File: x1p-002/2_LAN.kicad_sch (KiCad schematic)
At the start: 54 parts, among them U1 LAN9514, U5 M93C86-WMN6TP, X1 25MHz

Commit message: annotated everything with LCSC IDs
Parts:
- C10, C9: LCSC (none) -> C1557
- C12, C13, C14, C15, C16, C17, C18, C21, C22, C23, C24, C25, C26, C27, C28, C48: LCSC (none) -> C1525
- C29: LCSC (none) -> C52923
- R10, R12, R34: LCSC (none) -> C25744
- R11: footprint Capacitor_SMD:C_0402_1005Metric -> Resistor_SMD:R_0402_1005Metric; LCSC (none) -> C25752
- R28, R29, R31, R32, R33: LCSC (none) -> C17168
- R6: LCSC (none) -> C26083
- R8: LCSC (none) -> C25077
- TP4, TP5: now left out of the parts list
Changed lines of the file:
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@@
 			)
 		)
-		(property "Footprint" "Capacitor_SMD:C_0402_1005Metric"
+		(property "Footprint" "Resistor_SMD:R_0402_1005Metric"
 			(at 55.88 58.42 0)
 			(effects
@@
 			)
 		)
-		(property "LCSC" ""
+		(property "LCSC" "C25752"
 			(at 53.7718 54.4322 0)
 			(effects
@@
 			)
 		)
-		(property "LCSC" ""
+		(property "LCSC" "C1525"
 			(at 29.464 16.5608 0)
 			(effects
@@
 			)
 		)
-		(property "LCSC" ""
+		(property "LCSC" "C1525"
 			(at 53.1876 16.4084 0)
 			(effects
@@
 			)
 		)
-		(property "LCSC" ""
+		(property "LCSC" "C25744"
 			(at 54.61 123.5456 0)
 			(effects
@@
 			)
 		)
-		(property "LCSC" ""
+		(property "LCSC" "C1525"
 			(at 173.99 16.5608 0)
 			(effects
@@
 			)
 		)
-		(property "LCSC" ""
+		(property "LCSC" "C1557"
 			(at 23.876 91.7956 0)
 			(effects
@@
 			)
 		)
-		(property "LCSC" ""
+		(property "LCSC" "C1525"
 			(at 181.61 16.5608 0)
 			(effects
@@
 			)
 		)
-		(property "LCSC" ""
+		(property "LCSC" "C1525"
 			(at 189.23 16.5608 0)
 			(effects
@@
 			)
 		)
-		(property "LCSC" ""
+		(property "LCSC" "C52923"
 			(at 40.9956 55.4228 0)
 			(effects
@@
 			)
 		)
-		(property "LCSC" ""
+		(property "LCSC" "C17168"
 			(at 174.1889 182.88 0)
 			(effects
@@
 			)
 		)
-		(property "LCSC" ""
+		(property "LCSC" "C1525"
 			(at 219.71 173.3042 0)
 			(effects
@@
 		(unit 1)
 		(exclude_from_sim no)
-		(in_bom yes)
+		(in_bom no)
 		(on_board yes)
 		(dnp no)
@@
 			)
 		)
-		(property "LCSC" ""
+		(property "LCSC" "C1557"
 			(at 23.2156 74.0156 0)
 			(effects
@@
 			)
 		)
-		(property "LCSC" ""
+		(property "LCSC" "C26083"
 			(at 47.498 88.8238 0)
 			(effects
@@
 			)
 		)
-		(property "LCSC" ""
+		(property "LCSC" "C17168"
 			(at 154.94 152.5989 0)
 			(effects
@@
 			)
 		)
-		(property "LCSC" ""
+		(property "LCSC" "C1525"
 			(at 45.212 16.5608 0)
 			(effects
@@
 			)
 		)
-		(property "LCSC" ""
+		(property "LCSC" "C17168"
 			(at 57.15 129.7389 0)
 			(effects
@@
 			)
 		)
-		(property "LCSC" ""
+		(property "LCSC" "C25077"
 			(at 245.5926 24.257 0)
 			(effects
@@
 			)
 		)
-		(property "LCSC" ""
+		(property "LCSC" "C1525"
 			(at 196.85 16.5608 0)
 			(effects
@@
 			)
 		)
-		(property "LCSC" ""
+		(property "LCSC" "C1525"
 			(at 16.51 28.5242 0)
 			(effects
@@
 			)
 		)
-		(property "LCSC" ""
+		(property "LCSC" "C17168"
 			(at 57.15 142.0411 0)
 			(effects
@@
 			)
 		)
-		(property "LCSC" ""
+		(property "LCSC" "C17168"
 			(at 60.96 48.4589 0)
 			(effects
@@
 		(unit 1)
 		(exclude_from_sim no)
-		(in_bom yes)
+		(in_bom no)
 		(on_board yes)
 		(dnp no)
@@
 			)
 		)
-		(property "LCSC" ""
+		(property "LCSC" "C25744"
 			(at 167.8389 182.88 0)
 			(effects
@@
 			)
 		)
-		(property "LCSC" ""
+		(property "LCSC" "C1525"
 			(at 21.59 16.5608 0)
 			(effects
@@
 			)
 		)
-		(property "LCSC" ""
+		(property "LCSC" "C1525"
 			(at 158.75 16.5608 0)
 			(effects
@@
 			)
 		)
-		(property "LCSC" ""
+		(property "LCSC" "C1525"
 			(at 24.13 28.5242 0)
 			(effects
@@
 			)
 		)
-		(property "LCSC" ""
+		(property "LCSC" "C1525"
 			(at 151.13 16.5608 0)
 			(effects
@@
 			)
 		)
-		(property "LCSC" ""
+		(property "LCSC" "C1525"
 			(at 166.37 16.5608 0)
 			(effects
@@
 			)
 		)
-		(property "LCSC" ""
+		(property "LCSC" "C1525"
 			(at 40.64 40.9956 0)
 			(effects
@@
 			)
 		)
-		(property "LCSC" ""
+		(property "LCSC" "C1525"
 			(at 37.338 16.5608 0)
 			(effects
@@
 			)
 		)
-		(property "LCSC" ""
+		(property "LCSC" "C25744"
 			(at 54.9656 143.3576 0)
 			(effects

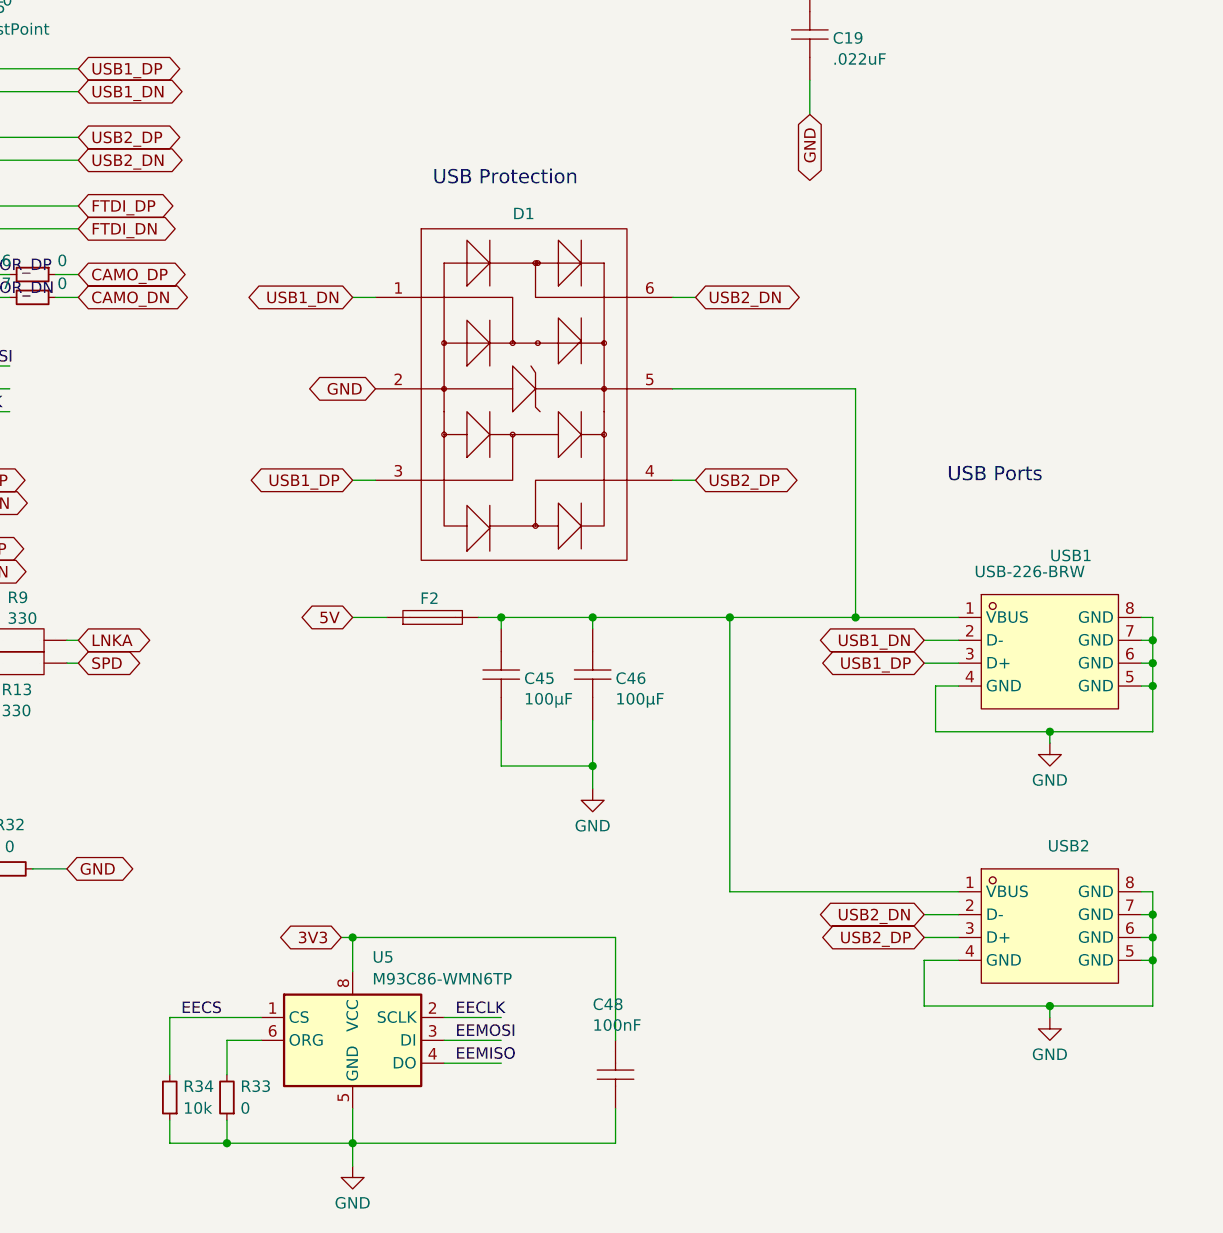
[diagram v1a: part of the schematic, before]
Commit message: stub-free usb esd protection
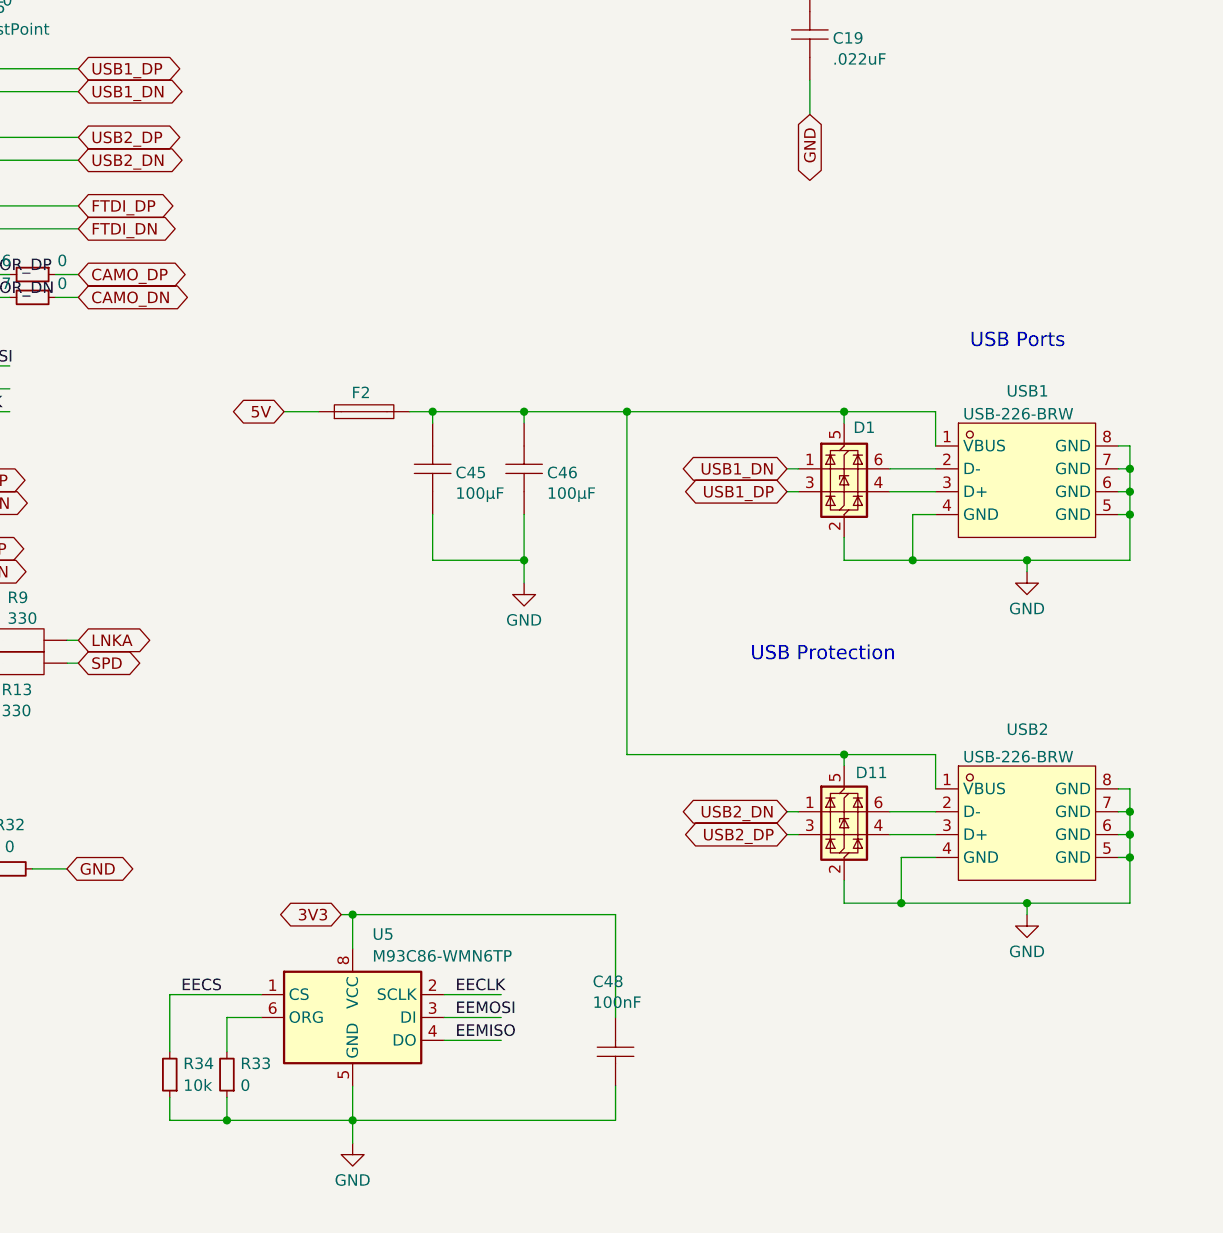
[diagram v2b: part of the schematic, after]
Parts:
- removed D1: SRV05-4.TCT_C2687126, x1-expander:SOT-23-6_L2.9-W1.6-P0.95-LS2.8-BL, symbol x1-expander:SRV05-4.TCT_C2687126
- added D1, D11: USBLC6-2SC6, Package_TO_SOT_SMD:SOT-23-6, symbol Power_Protection:USBLC6-2SC6
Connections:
- net GND: now also D1.2 (GND), D11.2 (GND)
- net USB1_DN: now also D1.1 (I/O1); no longer USB1.2 (D-)
- net USB1_DP: now also D1.3 (I/O2); no longer USB1.3 (D+)
- net USB2_DN: now also D11.1 (I/O1); no longer USB2.2 (D-)
- net USB2_DP: now also D11.3 (I/O2); no longer USB2.3 (D+)
- net at C45.2, C46.2, F2.2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: now also D1.5 (VBUS), D11.5 (VBUS)
- new net: D11.4 (I/O2), USB2.3 (D+)
- new net: D11.6 (I/O1), USB2.2 (D-)
- new net: D1.4 (I/O2), USB1.3 (D+)
- new net: D1.6 (I/O1), USB1.2 (D-)
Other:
- moved on the sheet: C45, C46, C48, F2, R33, R34, U5, USB1, USB2

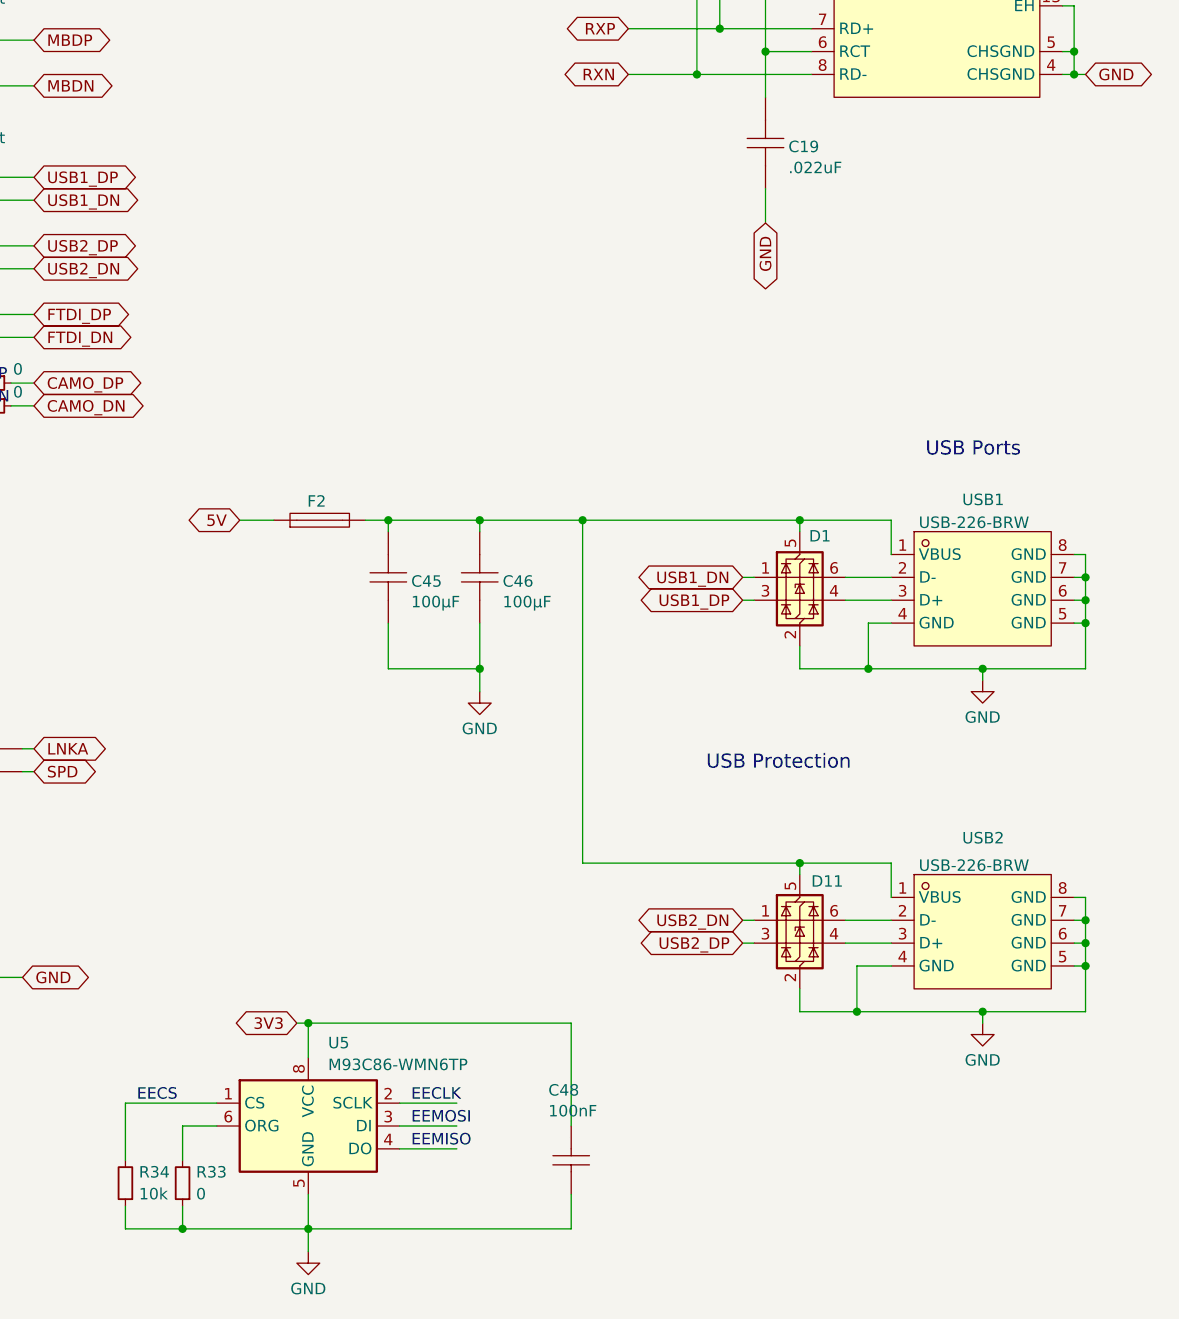
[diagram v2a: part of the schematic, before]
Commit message: implement esd double protection
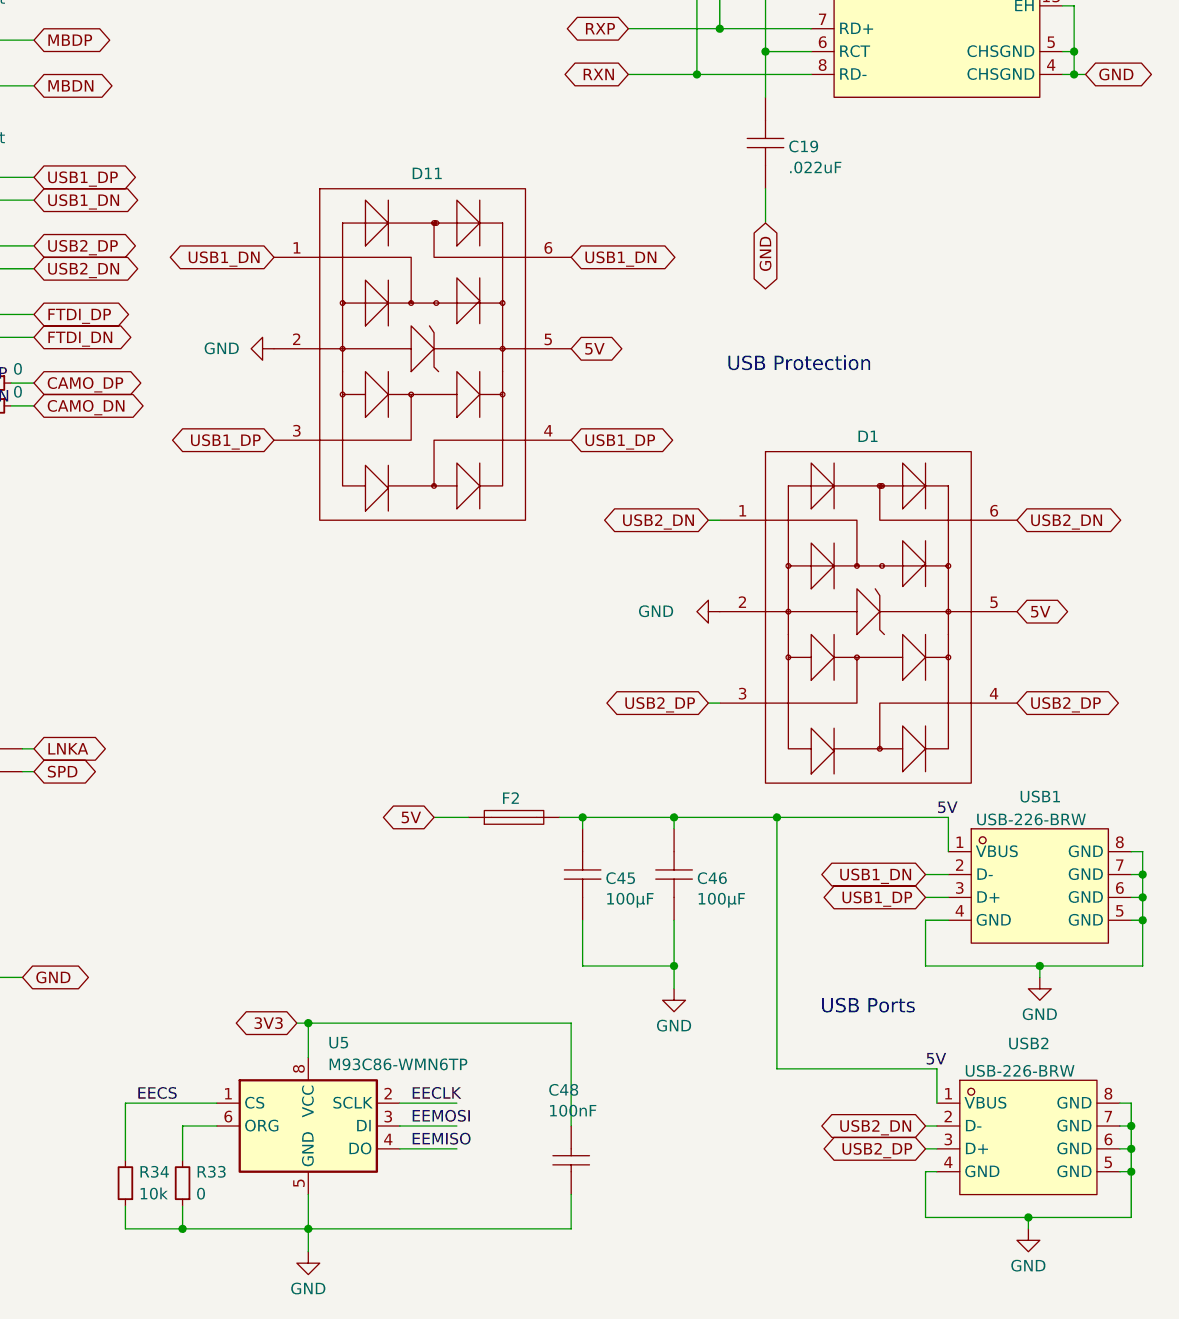
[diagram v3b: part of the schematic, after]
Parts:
- removed D1, D11: USBLC6-2SC6, Package_TO_SOT_SMD:SOT-23-6, symbol Power_Protection:USBLC6-2SC6
- added D1, D11: SRV05-4.TCT_C2687126, x1-expander:SOT-23-6_L2.9-W1.6-P0.95-LS2.8-BL, symbol x1-expander:SRV05-4.TCT_C2687126
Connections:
- net 5V: now also C45.2, C46.2, F2.2, USB1.1 (VBUS), USB2.1 (VBUS), D1.5, D11.5
- net GND: now also D1.2, D11.2
- net USB1_DN: now also USB1.2 (D-), D11.1, D11.6
- net USB1_DP: now also USB1.3 (D+), D11.3, D11.4
- net USB2_DN: now also USB2.2 (D-), D1.1, D1.6
- net USB2_DP: now also USB2.3 (D+), D1.3, D1.4
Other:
- moved on the sheet: C45, C46, F2, USB1, USB2
